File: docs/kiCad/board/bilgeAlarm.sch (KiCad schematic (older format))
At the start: 67 parts, among them J1 PUMP IN, J10 LCD_SDA, J11 LCD_SCL, J12 LCD_GND, J13 ALARM+, J14 ALARM-, J15 LED_GND, J16 LED_GND, J17 LED_DATA, J18 LED_DATA, J19 LED_5V, J2 PUMP2 IN, J20 LED_5V, J21 AUX, J22 AUX, J23 AUX, J24 AUX, J25 AUX, J26 AUX, J27 AUX, J28 AUX, J29 AUX, J3 PUMP OUT, J30 AUX, J31 AUX, J32 AUX, J33 AUX, J34 AUX, J35 AUX, J36 AUX, J37 AUX, J38 AUX, J39 AUX, J4 12V, J40 AUX, J41 AUX, J5 GND, J6 LED_5V, J7 LED_DATA, J8 LED_GND, J9 LCD_5V, K1 RELAY, M1 BUCK01, M2 SD_TYP0, Q1 IRLZ44N, Q2 BCS547, SW1 POWER, SW2 BUTTON1, SW3 BUTTON2, SW4 BUTTON3, U1 ESP32_DEV_0

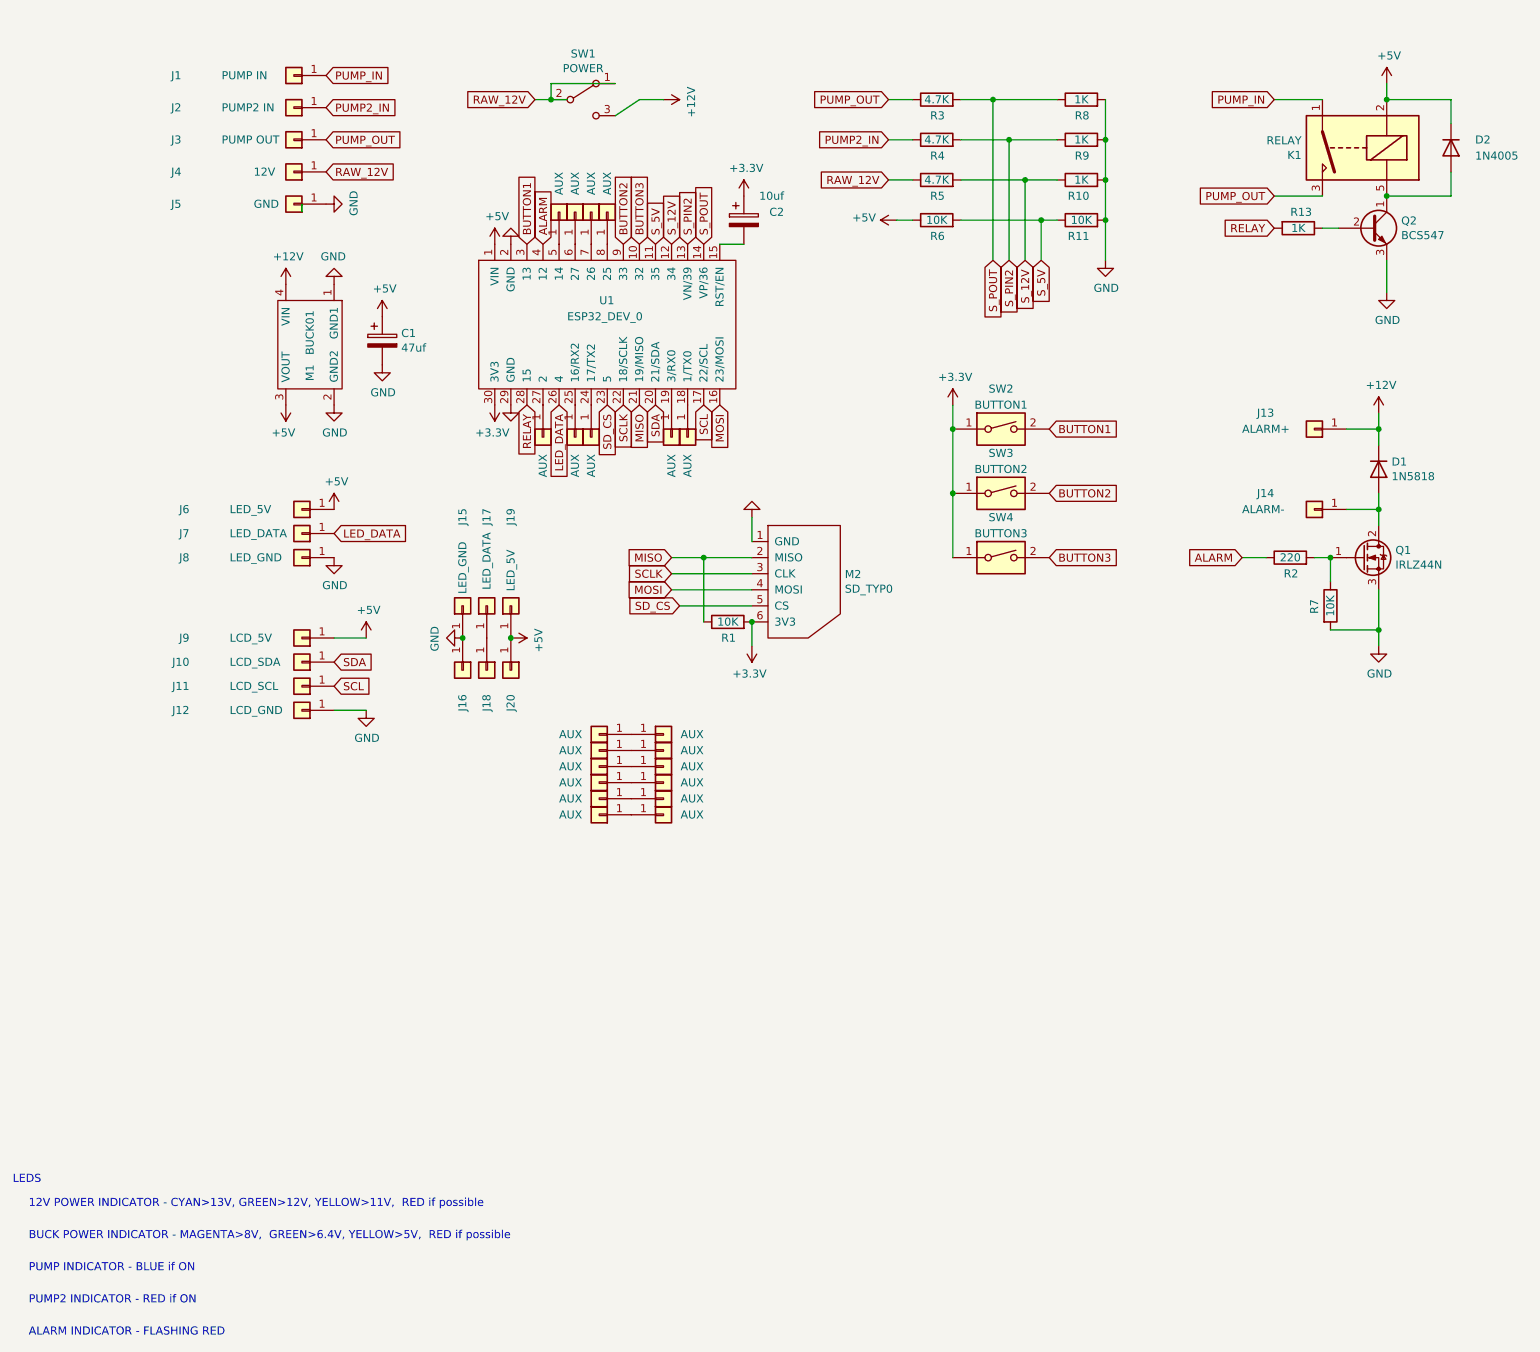
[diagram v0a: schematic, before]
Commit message: kicad - commit reworked PCB board using my new symbols and 3d footprints
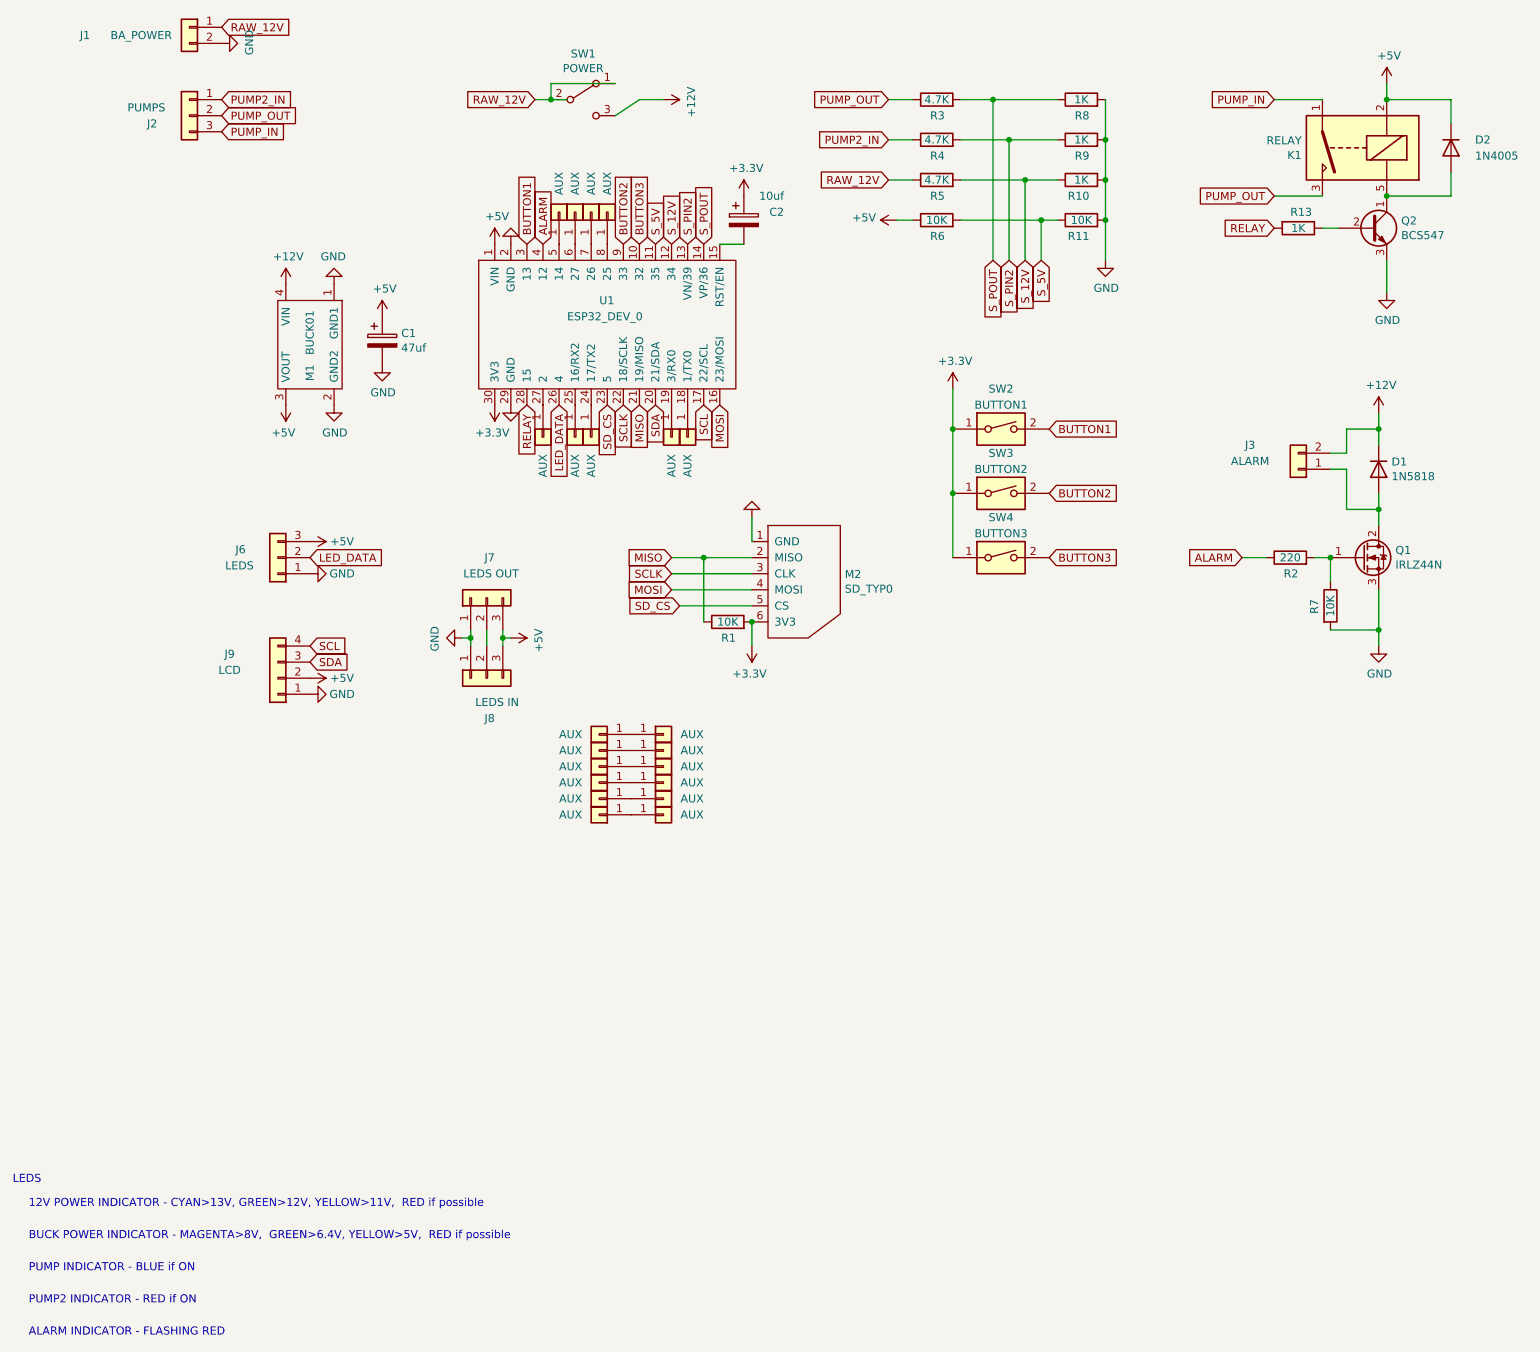
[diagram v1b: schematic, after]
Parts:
- removed J1: PUMP IN, cnc3018-PCB:my1pin, symbol Connector_Generic:Conn_01x01
- removed J10: LCD_SDA, cnc3018-PCB:my1pin, symbol Connector_Generic:Conn_01x01
- removed J11: LCD_SCL, cnc3018-PCB:my1pin, symbol Connector_Generic:Conn_01x01
- removed J12: LCD_GND, cnc3018-PCB:my1pin, symbol Connector_Generic:Conn_01x01
- removed J13: ALARM+, cnc3018-PCB:my1pin, symbol Connector_Generic:Conn_01x01
- removed J14: ALARM-, cnc3018-PCB:my1pin, symbol Connector_Generic:Conn_01x01
- removed J15, J16, J8: LED_GND, cnc3018-PCB:my1pin, symbol Connector_Generic:Conn_01x01
- removed J17, J18, J7: LED_DATA, cnc3018-PCB:my1pin, symbol Connector_Generic:Conn_01x01
- removed J19, J20, J6: LED_5V, cnc3018-PCB:my1pin, symbol Connector_Generic:Conn_01x01
- removed J2: PUMP2 IN, cnc3018-PCB:my1pin, symbol Connector_Generic:Conn_01x01
- removed J3: PUMP OUT, cnc3018-PCB:my1pin, symbol Connector_Generic:Conn_01x01
- removed J4: 12V, cnc3018-PCB:my1pin, symbol Connector_Generic:Conn_01x01
- removed J5: GND, cnc3018-PCB:my1pin, symbol Connector_Generic:Conn_01x01
- removed J9: LCD_5V, cnc3018-PCB:my1pin, symbol Connector_Generic:Conn_01x01
- added J1: BA_POWER, 0_my_footprints:myTerminalBlock_5.08x02, symbol Connector_Generic:Conn_01x02
- added J2: PUMPS, 0_my_footprints:myTerminalBlock_5.08x03, symbol Connector_Generic:Conn_01x03
- added J3: ALARM, 0_my_footprints:myTerminalBlock_5.08x02, symbol Connector_Generic:Conn_01x02
- added J6: LEDS, 0_my_footprints:myPinSocket_1x03, symbol Connector_Generic:Conn_01x03
- added J7: LEDS OUT, 0_my_footprints:myPinSocket_1x03, symbol Connector_Generic:Conn_01x03
- added J8: LEDS IN, 0_my_footprints:myPinSocket_1x03, symbol Connector_Generic:Conn_01x03
- added J9: LCD, 0_my_footprints:myPinSocket_1x04, symbol Connector_Generic:Conn_01x04
- C1: footprint cnc3018-PCB:my2pin -> 0_my_footprints:CP_my100uf
- C2: footprint cnc3018-PCB:my2pin -> 0_my_footprints:CP_my10uf
- D1, D2: footprint cnc3018-PCB:mySkip2 -> 0_my_footprints:myDiodeSchotsky
- K1: footprint Relay_THT:Relay_SPDT_SANYOU_SRD_Series_Form_C -> 0_my_footprints:myRelay
- M1: footprint cnc3018-PCB:BUCK01 -> 0_my_footprints:myMini360BuckConverter
- M2: footprint cnc3018-PCB:my6Pin -> 0_my_footprints:SDCardReader
- Q1: footprint Package_TO_SOT_THT:TO-220-3_Vertical -> 0_my_footprints:myTO-220-3
- R1, R10, R11, R13, R2, R3, R4, R5, R6, R7, R8, R9: footprint cnc3018-PCB:myResistor -> 0_my_footprints:myResistor
- SW1: footprint cnc3018-PCB:SW_DPDT_BLUE_LEVER -> 0_my_footprints:mySwitchToggleSPDT
- SW2, SW3, SW4: footprint cnc3018-PCB:BUTTON -> 0_my_footprints:myButton
- U1: footprint cnc3018-PCB:ESP32-DEV_0 -> 0_my_footprints:myESP32DEV0
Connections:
- wire segments 62 -> 70
